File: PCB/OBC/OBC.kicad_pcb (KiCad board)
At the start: 2 copper layers, 81 x 81 mm, 127 parts, among them IC1 TPS2553QDBVRQ1, J1 Conn_02x24_Odd_Even, J3 USB_C_Receptacle_USB2.0_16P, U1 STM32F405RGTx, U10 TMUX1574PWR, U11 W25Q128JVSIQ, U12 SN65HVD230DR, U2 SN65HVD230DR, U3 USBLC6-2SC6, U4 STM32F405RGTx, U5 STM32F405RGTx, U6 MAX6369KA+T, U7 AMS1117-3.3, U8 TMUX1574PWR, U9 W25Q128JVSIQ

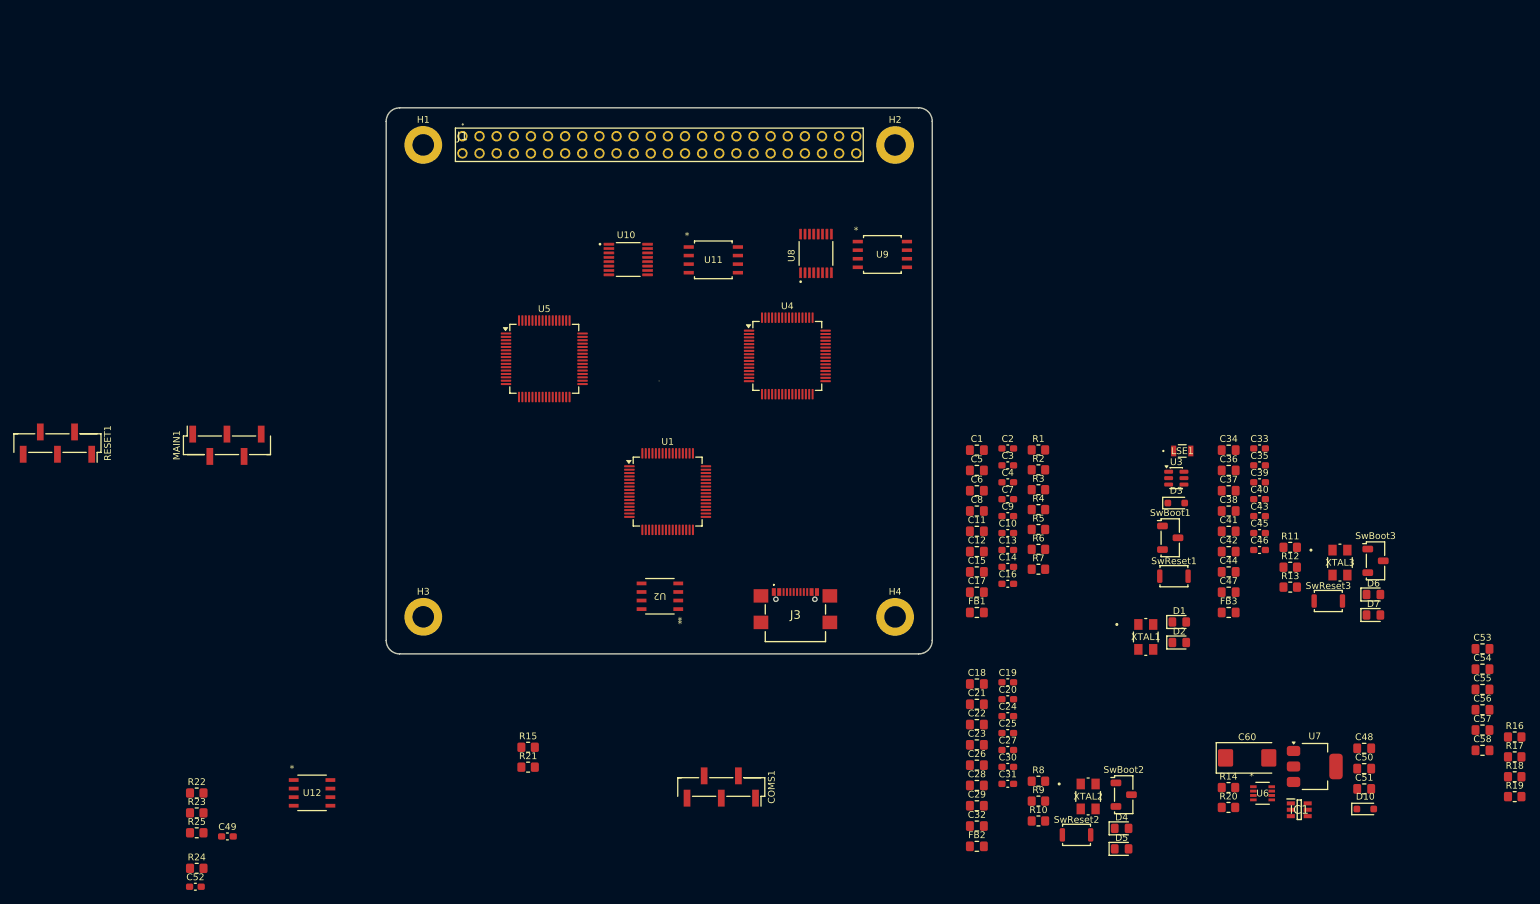
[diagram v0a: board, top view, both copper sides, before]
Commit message: Placement
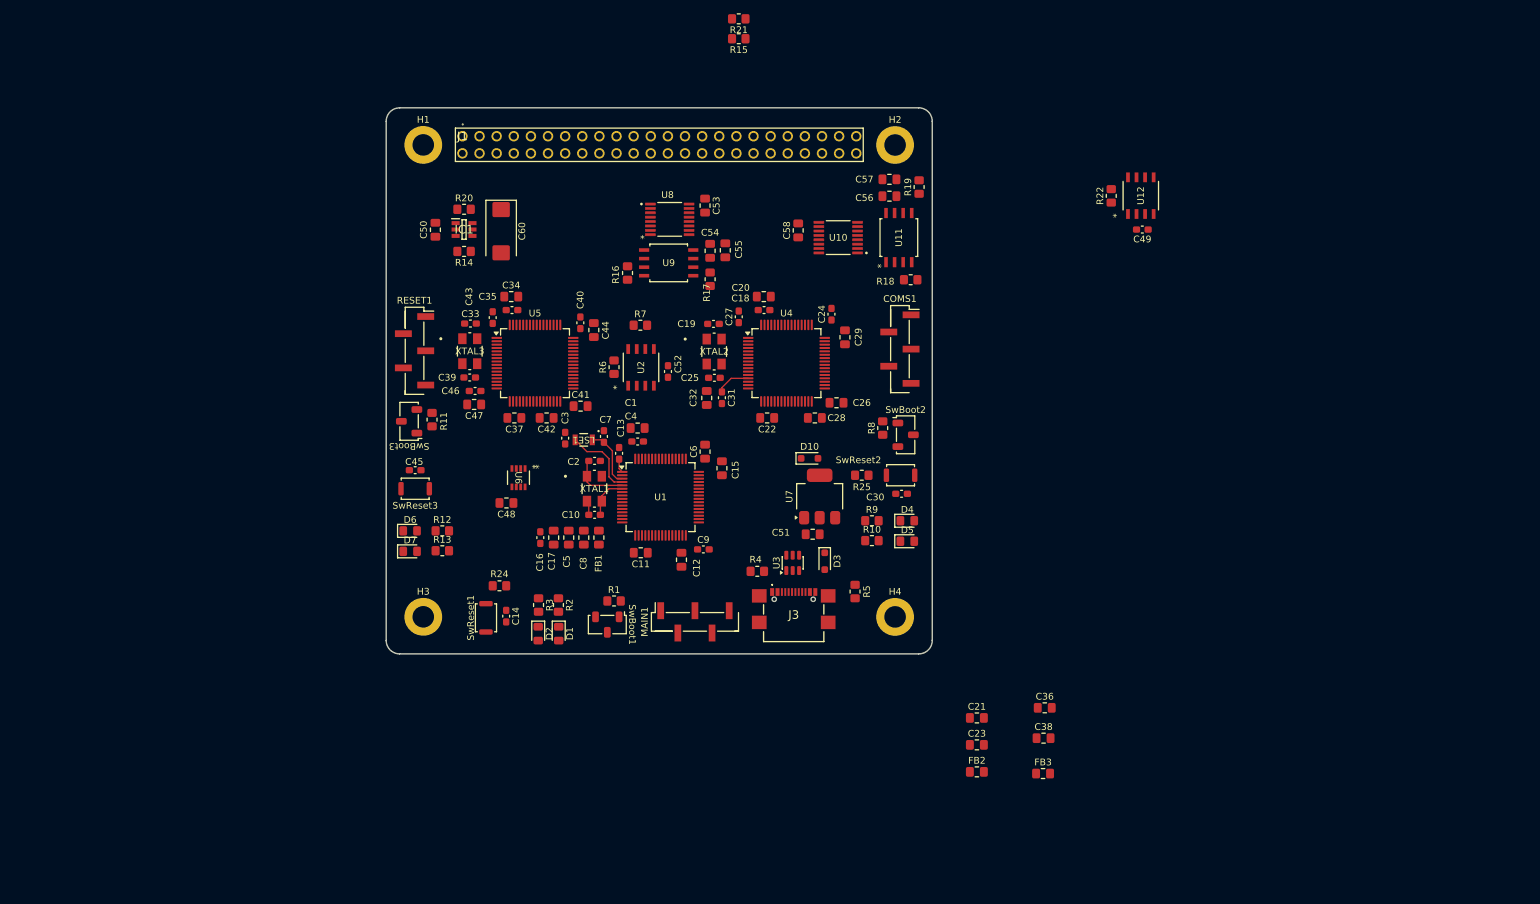
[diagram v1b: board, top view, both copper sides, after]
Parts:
- removed R23: 120, Resistor_SMD:R_0805_2012Metric_Pad1.20x1.40mm_HandSolder
- moved C49 162.9 mm to (222.4, 62.6), turned to 180 degrees
- moved R22 162.0 mm to (217.8, 57.6), turned to 90 degrees
- moved C50 159.3 mm to (117.5, 62.6), turned to -90 degrees
- moved U12 151.5 mm to (222.1, 57.5), turned to 90 degrees
- moved IC1 150.9 mm to (121.8, 62.5)
- moved R16 148.5 mm to (146.0, 69.0), turned to -90 degrees
- moved SwBoot3 144.8 mm to (113.6, 91.0), turned to 180 degrees
- moved R20 144.0 mm to (121.8, 59.5)
- moved D6 143.2 mm to (113.8, 107.2)
- moved D7 143.2 mm to (113.8, 110.3)
- moved R17 138.8 mm to (158.2, 69.9), turned to -90 degrees
- moved R14 138.5 mm to (121.8, 65.8), turned to 180 degrees
- moved SwReset3 136.5 mm to (114.5, 101.0)
- moved C60 135.5 mm to (127.2, 62.8), turned to -90 degrees
- moved XTAL3 132.8 mm to (122.6, 80.6)
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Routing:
- net /Main/LSE_OUT: track 0.00 -> 11.2 mm
- net /Main/LSE_IN: track 0.00 -> 8.87 mm
- net /Main/HSE_IN: track 0.00 -> 8.67 mm
- net /Main/HSE_OUT: track 0.00 -> 6.37 mm
- net +3V3A: track 0.00 -> 5.11 mm
- net GND: track 0.00 -> 2.13 mm
- net +3V3: track 0.00 -> 2.08 mm
- added copper zone on In1.Cu, net GND
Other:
- copper layers 2 -> 4

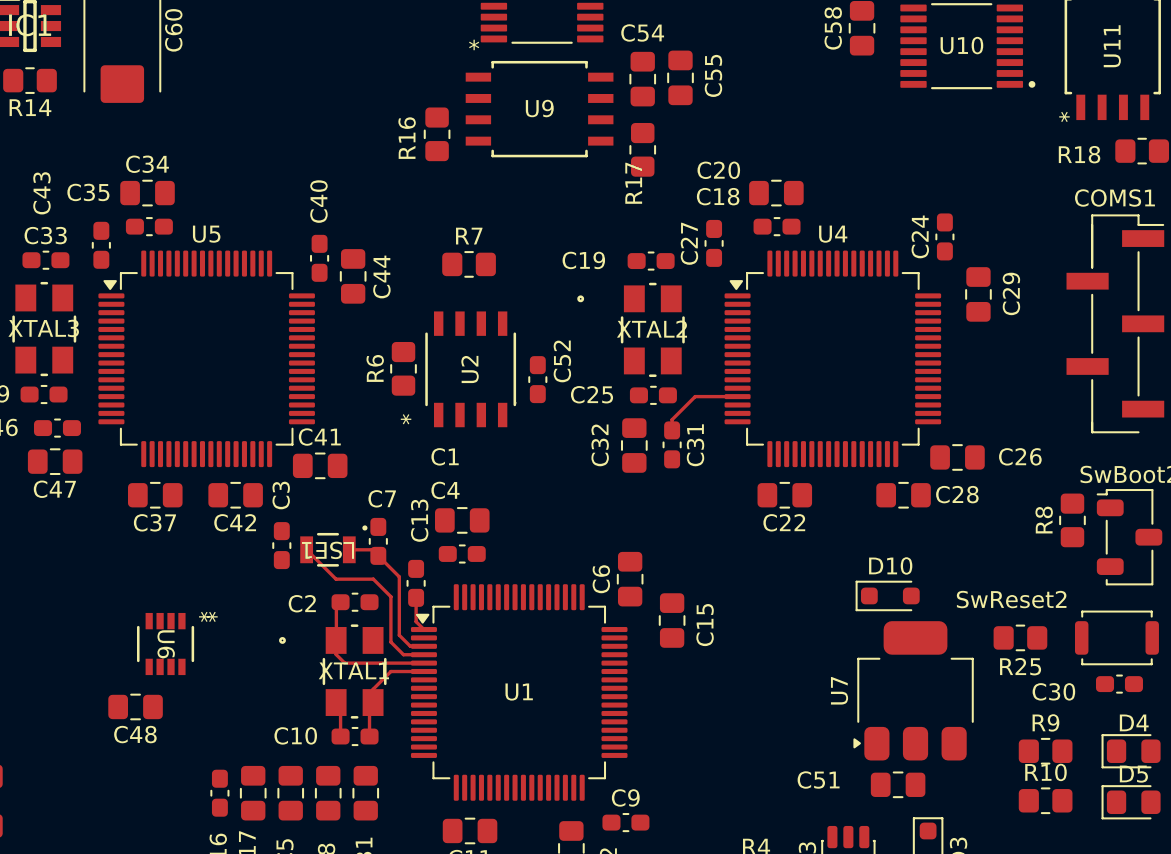
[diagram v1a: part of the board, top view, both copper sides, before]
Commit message: PC104
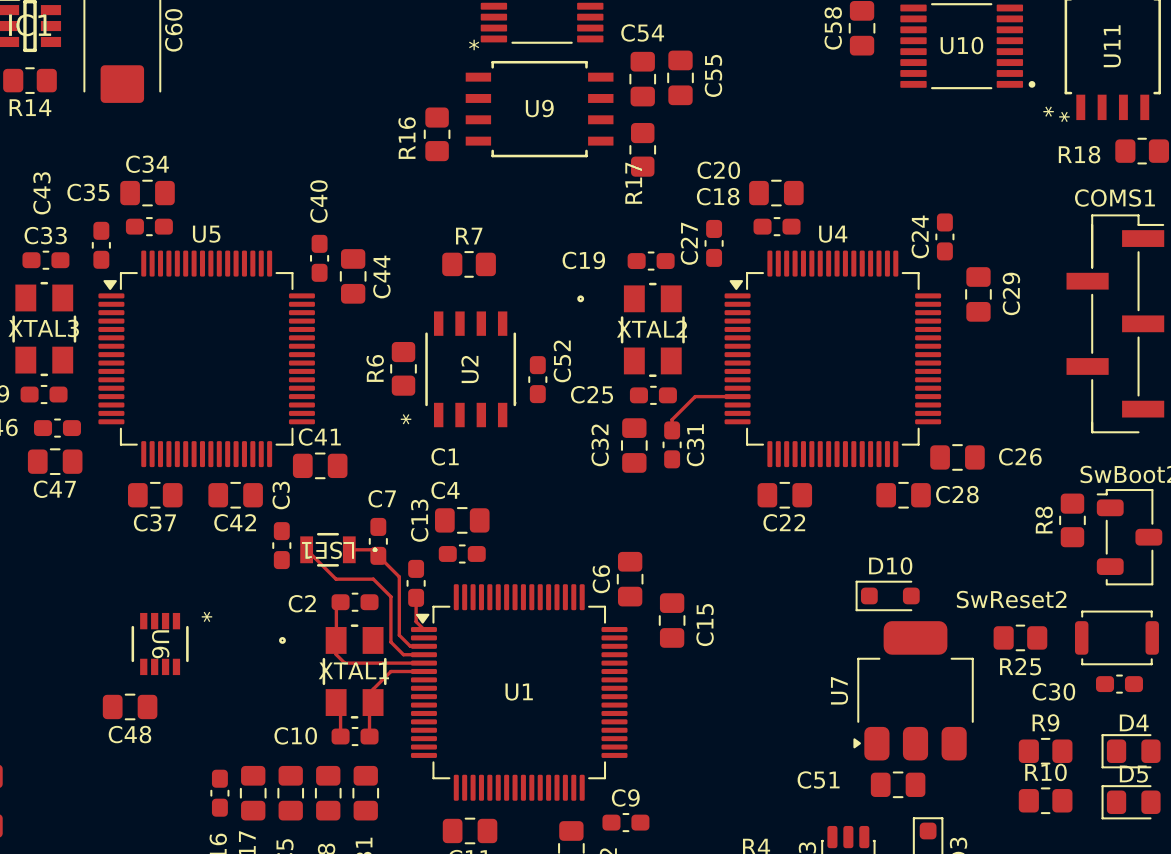
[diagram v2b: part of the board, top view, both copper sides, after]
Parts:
- moved C48 0.33 mm to (127.7, 103.1)
- moved U6 0.33 mm to (129.5, 99.4)
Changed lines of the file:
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@@
 	)
 	(footprint "ESQ-124-38-L-D:ESQ-124-Y-X-D"
+		(locked yes)
 		(layer "F.Cu")
 		(at 121.506655 48.713416 180)
@@
 			)
 		)
-		(fp_text user "*"
-			(at -1.6129 -2.4257 90)
+		(fp_text user "${REFERENCE}"
+			(at 0 0 90)
+			(unlocked yes)
 			(layer "F.Fab")
 			(effects
@@
 			)
 		)
-		(fp_text user "${REFERENCE}"
-			(at 0 0 90)
-			(unlocked yes)
+		(fp_text user "*"
+			(at -1.6129 -2.4257 90)
 			(layer "F.Fab")
 			(effects
@@
 		)
 		(embedded_fonts no)
+		(model "${KIPRJMOD}/assets/ul_SN65HVD230DR/D0008A.stp"
+			(offset
+				(xyz 0 0 0)
+			)
+			(scale
+				(xyz 1 1 1)
+			)
+			(rotate
+				(xyz 0 0 0)
+			)
+		)
 	)
 	(footprint "Capacitor_SMD:C_0805_2012Metric_Pad1.18x1.45mm_HandSolder"
@@
 	(footprint "Capacitor_SMD:C_0805_2012Metric_Pad1.18x1.45mm_HandSolder"
 		(layer "F.Cu")
-		(at 128.037501 103.113149 180)
+		(at 127.7125 103.113149 180)
 		(descr "Capacitor SMD 0805 (2012 Metric), square (rectangular) end terminal, IPC-7351 nominal with elongated pad for handsoldering. (Body size source: IPC-SM-782 page 76, https://www.pcb-3d.com/wordpress/wp-content/uploads/ipc-sm-782a_amendment_1_and_2.pdf, https://docs.google.com/spreadsheets/d/1BsfQQcO9C6DZCsRaXUlFlo91Tg2WpOkGARC1WS5S8t0/edit?usp=sharing), generated with kicad-footprint-generator")
 		(tags "capacitor handsolder")
@@
 		)
 		(fp_circle
-			(center -2.2 1.3)
-			(end -2.1238 1.3)
+			(center -2.8067 0)
+			(end -2.7305 0)
 			(stroke
 				(width 0.1524)
@@
 	(footprint "MAX6369KA+T:21-0078H_MXM"
 		(layer "F.Cu")
-		(at 129.825001 99.363149 -90)
+		(at 129.5 99.363149 -90)
 		(tags "MAX6369KA+T ")
 		(property "Reference" "U6"
@@
 		)
 		(fp_text user "*"
-			(at -1.617149 -2.549 90)
+			(at -1.617149 -2.549 270)
+			(unlocked yes)
 			(layer "F.SilkS")
 			(effects
@@
 		)
 		(fp_text user "*"
-			(at -0.4953 -1.4224 90)
+			(at -0.4953 -1.4224 270)
+			(unlocked yes)
 			(layer "F.Fab")
 			(effects
@@
 		)
 		(embedded_fonts no)
+		(model "${KIPRJMOD}/assets/TMUX1574PWR/TMUX1574PWR.step"
+			(offset
+				(xyz 0 0 0)
+			)
+			(scale
+				(xyz 1 1 1)
+			)
+			(rotate
+				(xyz -90 -0 -0)
+			)
+		)
 	)
 	(footprint "Resistor_SMD:R_0805_2012Metric_Pad1.20x1.40mm_HandSolder"
@@
 		)
 		(fp_text user "*"
-			(at -4.2141 -2.6356 90)
+			(at -3.8989 -3.5806 90)
 			(layer "F.SilkS")
 			(effects
@@
 		(fp_text user "*"
 			(at -2.286 -2.5908 90)
+			(unlocked yes)
 			(layer "F.Fab")
 			(effects
@@
 		)
 		(embedded_fonts no)
-		(model "${KIPRJMOD}/Footprints/ul_W25Q128JVSIQ/SOIC_128JVSIQ_WIN.step"
+		(model "${KIPRJMOD}/assets/ul_W25Q128JVSIQ/SOIC_128JVSIQ_WIN.step"
 			(offset
 				(xyz 0 0 0)
@@
 		)
 		(embedded_fonts no)
+		(model "${KIPRJMOD}/assets/TMUX1574PWR/TMUX1574PWR.step"
+			(offset
+				(xyz 0 0 0)
+			)
+			(scale
+				(xyz 1 1 1)
+			)
+			(rotate
+				(xyz -90 -0 -0)
+			)
+		)
 	)
 	(footprint "OCP_TPS2553QDBVRQ1:SOT95P280X145-6N"
@@
 		(fp_text user "*"
 			(at -2.286 -2.5908 0)
-			(unlocked yes)
 			(layer "F.Fab")
 			(effects
@@
 			)
 		)
-		(fp_text user "*"
-			(at -2.286 -2.5908 0)
+		(fp_text user "${REFERENCE}"
+			(at 0 0 0)
+			(unlocked yes)
 			(layer "F.Fab")
 			(effects
@@
 			)
 		)
-		(fp_text user "${REFERENCE}"
-			(at 0 0 0)
+		(fp_text user "*"
+			(at -2.286 -2.5908 0)
 			(unlocked yes)
 			(layer "F.Fab")
@@
 		)
 		(embedded_fonts no)
-		(model "${KIPRJMOD}/Footprints/ul_W25Q128JVSIQ/SOIC_128JVSIQ_WIN.step"
+		(model "${KIPRJMOD}/assets/ul_W25Q128JVSIQ/SOIC_128JVSIQ_WIN.step"
 			(offset
 				(xyz 0 0 0)
@@
 		(fp_text user "*"
 			(at -2.97535 -3.606 90)
-			(unlocked yes)
 			(layer "F.SilkS")
 			(effects
@@
 		)
 		(embedded_fonts no)
+		(model "${KIPRJMOD}/assets/ul_SN65HVD230DR/D0008A.stp"
+			(offset
+				(xyz 0 0 0)
+			)
+			(scale
+				(xyz 1 1 1)
+			)
+			(rotate
+				(xyz 0 0 0)
+			)
+		)
 	)
 	(gr_line
